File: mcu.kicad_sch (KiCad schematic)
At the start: 18 parts, among them CN1 HX JN1.27-2X5 TP H4.9, SW1 TS-1088-AR02016, U1 STM32F405RGTx, U6 SS12D10G5

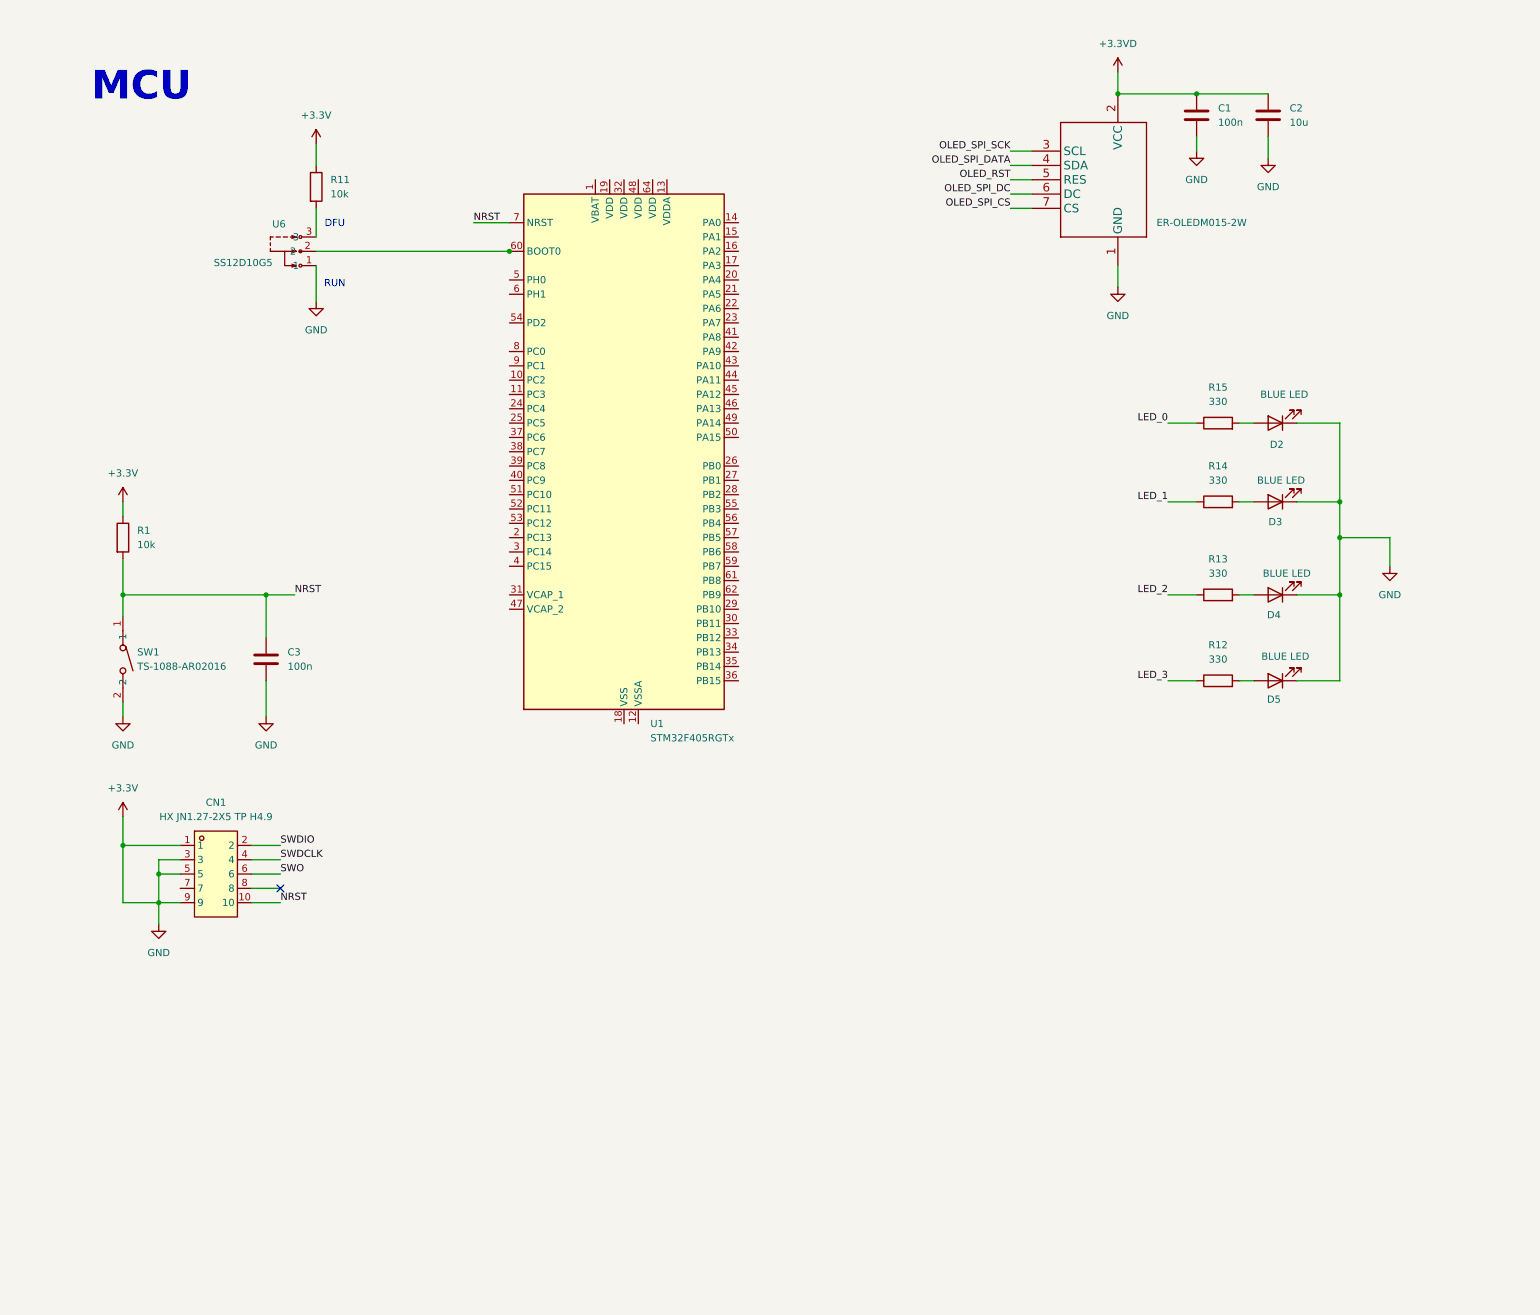
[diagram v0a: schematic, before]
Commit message: First pins assingments
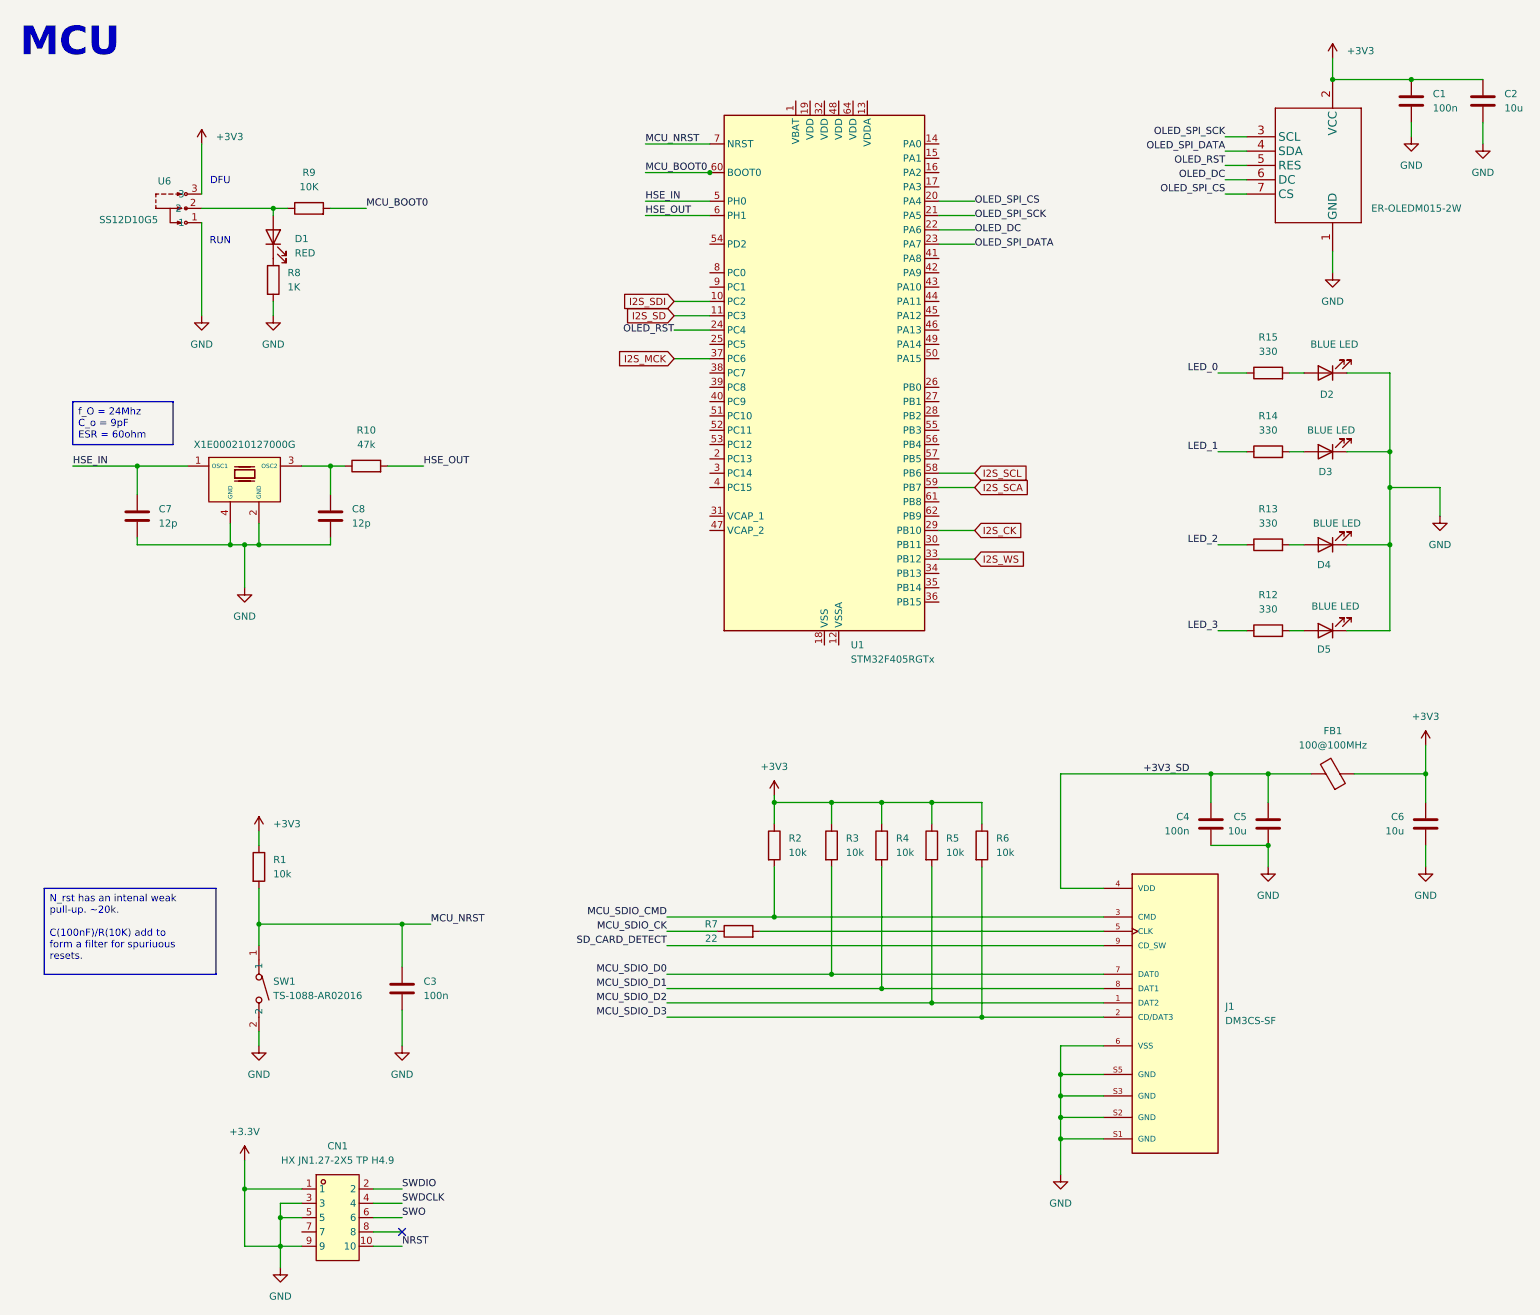
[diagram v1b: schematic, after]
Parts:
- removed R11: 10k, symbol Device:R
- added C4: 100n, symbol Device:C
- added C5, C6: 10u, symbol Device:C
- added C7, C8: 12p, symbol Device:C
- added D1: RED, symbol Device:LED
- added FB1: 100@100MHz, symbol Device:FerriteBead
- added J1: DM3CS-SF, Galerna:HRS_DM3CS-SF, symbol Galerna:DM3CS-SF
- added R10: 47k, symbol Device:R
- added R2, R3, R4, R5, R6: 10k, symbol Device:R
- added R7: 22, symbol Device:R
- added R8: 1K, symbol Device:R
- added R9: 10K, symbol Device:R
- added X1: X1E000210127000G, Galerna:CRYSTAL-SMD_4P-L3.2-W2.5-BL, symbol Galerna:X1E000210127000G
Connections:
- net +3.3VD is gone; now on net +3V3: C1.1, C2.1, ER-OLEDM015-2W.2 (VCC)
- net OLED_SPI_DC is gone; now on net OLED_DC: ER-OLEDM015-2W.6 (DC)
- net +3.3V: now also C4.2, C5.2, C6.2, C7.2, C8.2, J1.6 (VSS), J1.S1 (GND), J1.S2 (GND), J1.S3 (GND), J1.S5 (GND), R8.2, X1.2 (GND), X1.4 (GND); no longer R1.1
- net NRST: no longer C3.1, R1.2, SW1.1, U1.7 (NRST)
- net OLED_RST: now also U1.24 (PC4)
- net OLED_SPI_CS: now also U1.20 (PA4)
- net OLED_SPI_DATA: now also U1.23 (PA7)
- net OLED_SPI_SCK: now also U1.21 (PA5)
- net at U6.2: now also D1.2 (A), R9.1; no longer U1.60 (BOOT0)
- net +3V3: now reaches U6.3
- net +3V3: now also R1.1, C6.1, FB1.1, R2.1, R3.1, R4.1, R5.1, R6.1
- net I2S_SDI: now reaches U1.10 (PC2)
- net I2S_SD: now reaches U1.11 (PC3)
- net OLED_DC: now reaches U1.22 (PA6)
- net I2S_CK: now reaches U1.29 (PB10)
- net I2S_WS: now reaches U1.33 (PB12)
- net I2S_MCK: now reaches U1.37 (PC6)
- net HSE_IN: now reaches U1.5 (PH0)
- net HSE_IN: now also C7.1, X1.1 (OSC1)
- net I2S_SCL: now reaches U1.58 (PB6)
- net I2S_SCA: now reaches U1.59 (PB7)
- net HSE_OUT: now reaches U1.6 (PH1)
- net HSE_OUT: now also R10.2
- new net: C8.1, R10.1, X1.3 (OSC2)
- new net: D1.1 (K), R8.1
- new net: J1.5 (CLK), R7.2
- new net +3V3_SD: C4.1, C5.1, FB1.2, J1.4 (VDD)
- new net MCU_BOOT0: R9.2, U1.60 (BOOT0)
- new net MCU_NRST: C3.1, R1.2, SW1.1, U1.7 (NRST)
- new net MCU_SDIO_CK: R7.1
- new net MCU_SDIO_CMD: J1.3 (CMD), R2.2
- new net MCU_SDIO_D0: J1.7 (DAT0), R3.2
- new net MCU_SDIO_D1: J1.8 (DAT1), R4.2
- new net MCU_SDIO_D2: J1.1 (DAT2), R5.2
- new net MCU_SDIO_D3: J1.2 (CD/DAT3), R6.2
- new net SD_CARD_DETECT: J1.9 (CD_SW)
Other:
- moved on the sheet: C1, C2, C3, CN1, D2, D3, D4, D5, ER-OLEDM015-2W, R1, R12, R13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

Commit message: MCU connected
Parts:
- removed D5: BLUE LED, symbol Device:LED
- removed R12: 330, symbol Device:R
- added C23, C24, C25, C26, C27: 100n, symbol Device:C
- added C28: 10u, symbol Device:C
- added C29: 10n, symbol Device:C
- added C30, C31: 1u, symbol Device:C
- added C32, C33: 2.2, symbol Device:C
- added L2: 10n, symbol Device:L
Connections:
- net +3.3V is gone; now on net +3V3: C1.2, C2.2, C3.2, C4.2, C5.2, C6.2, C7.2, C8.2, CN1.1, CN1.3, CN1.5, CN1.9, D2.1 (K), D3.1 (K), D4.1 (K), ER-OLEDM015-2W.1 (GND), J1.6 (VSS), J1.S1 (GND), J1.S2 (GND), J1.S3 (GND), J1.S5 (GND), R8.2, SW1.2, U6.1, X1.2 (GND), X1.4 (GND)
- net NRST is gone; now on net MCU_NRST: CN1.10
- net +3V3: now also U1.1 (VBAT), U1.12 (VSSA), U1.18 (VSS), U1.19 (VDD), U1.32 (VDD), U1.48 (VDD), U1.63 (VSS), U1.64 (VDD), C23.1, C23.2, C24.1, C24.2, C25.1, C25.2, C26.1, C26.2, C27.1, C27.2, C28.1, C28.2, C29.2, C30.2, C31.1, C31.2, C32.2, C33.2, L2.2
- net HSE_IN: no longer U1.5 (PH0)
- net HSE_OUT: no longer U1.6 (PH1)
- net LED_0: now also U1.43 (PA10)
- net LED_1: now also U1.42 (PA9)
- net LED_2: now also U1.41 (PA8)
- net MCU_BOOT0: no longer U1.60 (BOOT0)
- net MCU_SDIO_CK: now also U1.53 (PC12)
- net MCU_SDIO_CMD: now also U1.54 (PD2)
- net MCU_SDIO_D0: now also U1.39 (PC8)
- net MCU_SDIO_D1: now also U1.40 (PC9)
- net MCU_SDIO_D2: now also U1.51 (PC10)
- net MCU_SDIO_D3: now also U1.52 (PC11)
- net SD_CARD_DETECT: now also U1.50 (PA15)
- net SWDCLK: now also U1.49 (PA14)
- net SWDIO: now also U1.46 (PA13)
- net SWO: now also U1.55 (PB3)
- net at U1.13 (VDDA): now also C29.1, C30.1, L2.1
- net POT_MUX_ADC: now reaches U1.14 (PA0)
- net POT_MUX_SEL_2: now reaches U1.26 (PB0)
- net POT_MUX_SEL_1: now reaches U1.27 (PB1)
- net POT_MUX_SEL_0: now reaches U1.28 (PB2)
- net at U1.31 (VCAP_1): now also C33.1
- net MCU_USB_D-: now reaches U1.44 (PA11)
- net MCU_USB_D+: now reaches U1.45 (PA12)
- net at U1.47 (VCAP_2): now also C32.1
- new net MCU_HSE_IN: U1.5 (PH0)
- new net MCU_HSE_OUT: U1.6 (PH1)
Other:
- note added: "MCU_VCAP_1"
- note added: "MCU_VCAP_2"
- moved on the sheet: C1, C2, C3, C4, C5, C6, CN1, D2, D3, D4, ER-OLEDM015-2W, FB1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
